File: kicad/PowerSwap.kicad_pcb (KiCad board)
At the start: 2 copper layers, 19 parts, among them U1 TPS63030

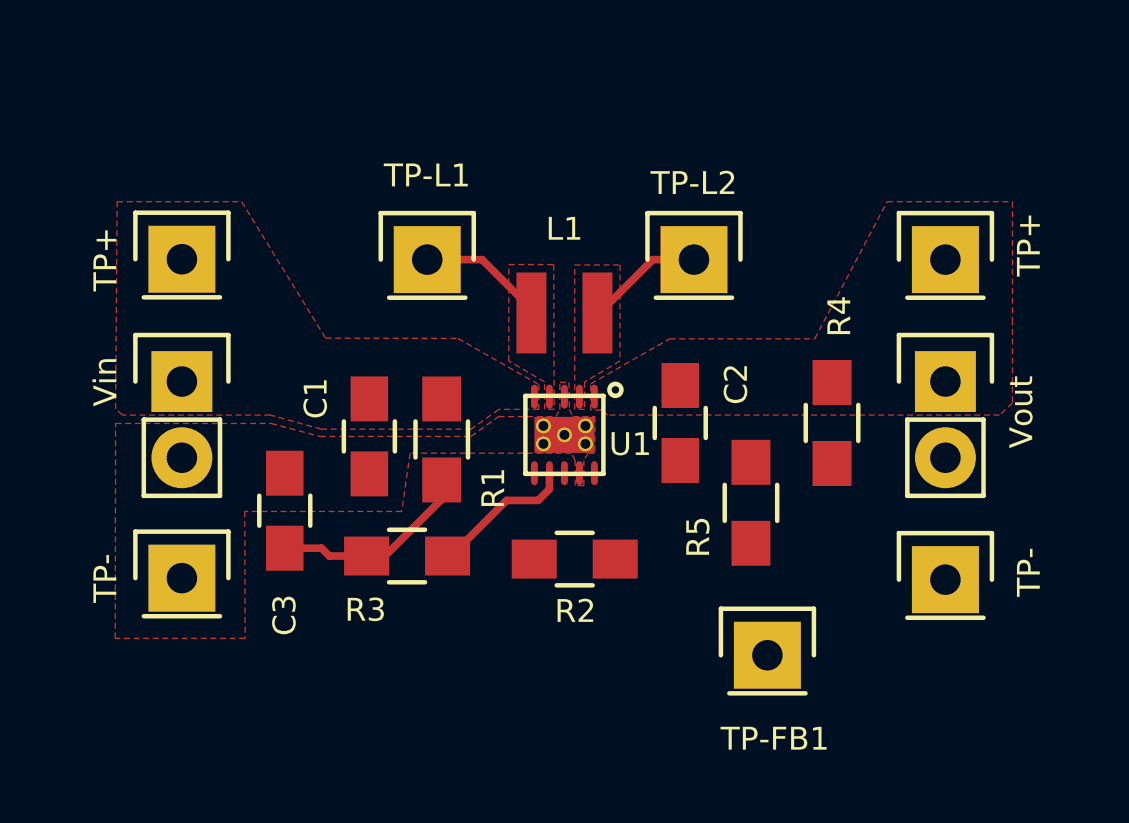
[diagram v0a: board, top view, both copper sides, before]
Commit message: Completed layout
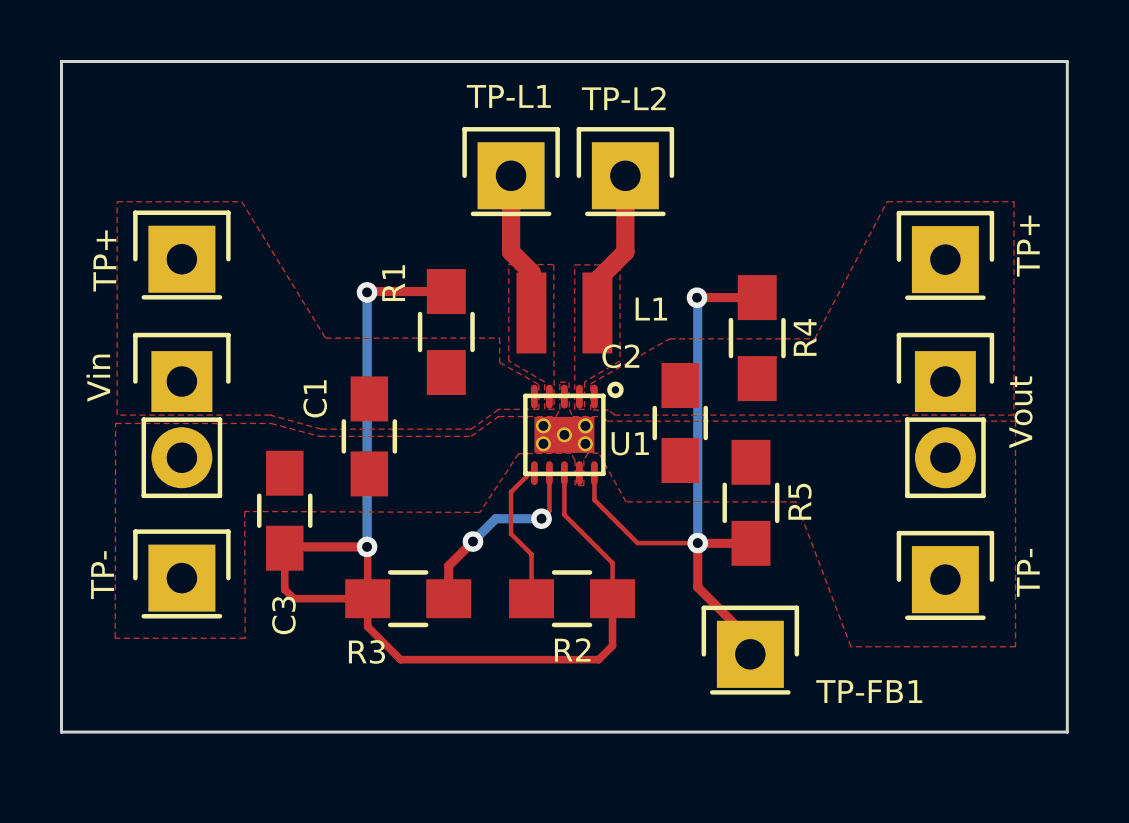
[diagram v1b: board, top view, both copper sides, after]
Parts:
- moved TP-L1 3.95 mm to (144.0, 86.1)
- moved R4 3.77 mm to (152.2, 91.5), turned to 90 degrees
- moved TP-L2 3.61 mm to (147.8, 86.1)
- moved R1 3.58 mm to (141.9, 91.3), turned to 270 degrees
- moved R3 1.42 mm to (140.6, 100.2)
- moved R2 1.32 mm to (146.1, 100.2)
- moved TP-FB1 0.57 mm to (152.0, 102.1)
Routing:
- net Net-(C3-Pad1): track 6.81 -> 36.3 mm, vias 0 -> 2
- net /Feedback: track 0.01 -> 21.4 mm, vias 0 -> 2
- net Net-(R2-Pad1): track 0.00 -> 4.89 mm
- net Net-(R3-Pad1): track 4.85 -> 6.47 mm, vias 0 -> 2
- net Net-(L1-Pad2): track 3.95 -> 5.03 mm
- net Net-(L1-Pad1): track 4.29 -> 5.05 mm
- added copper zone on B.Cu, net GNDPWR
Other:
- board outline added: 33.5 x 22.4 mm

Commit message: Final layout
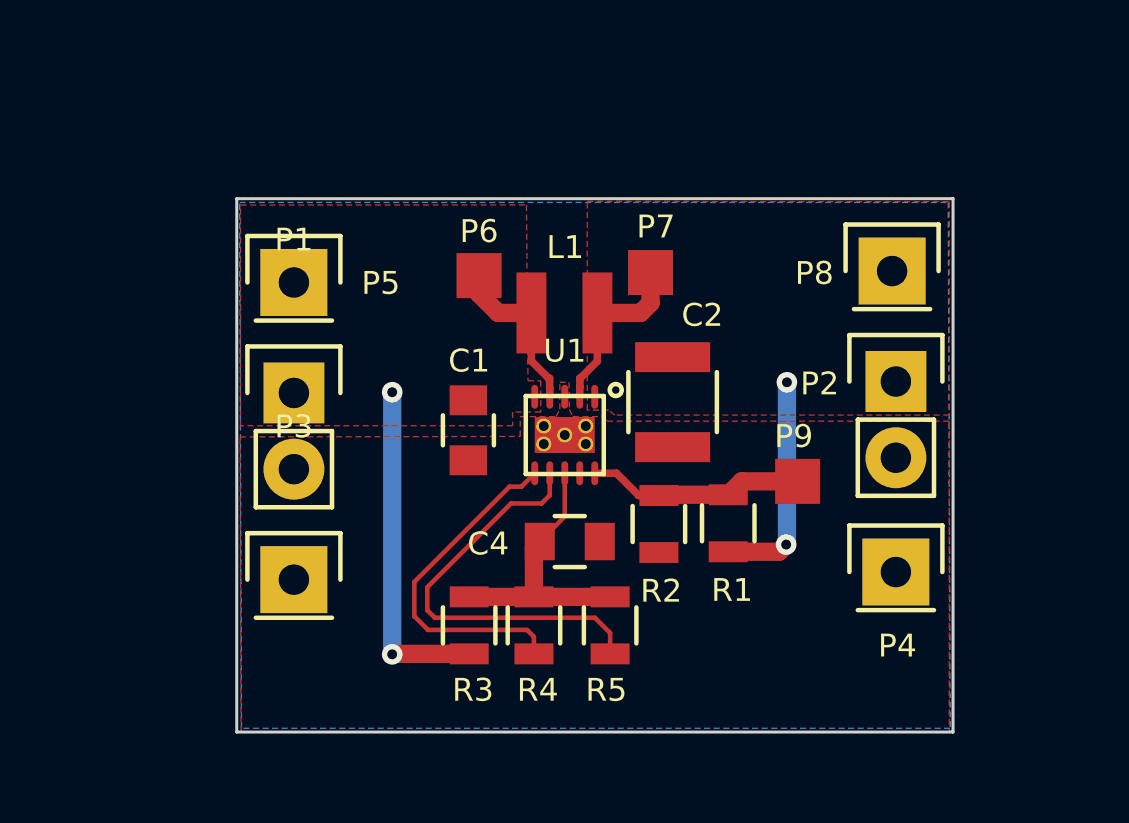
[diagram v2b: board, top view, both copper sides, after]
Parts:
- removed C3: 0.1μF, Capacitors_SMD:C_0805_HandSoldering
- removed TP+: Vin, Pin_Headers:Pin_Header_Straight_1x01
- removed TP+: Vout, Pin_Headers:Pin_Header_Straight_1x01
- removed TP-: GND, Pin_Headers:Pin_Header_Straight_1x01
- removed TP-: PGND, Pin_Headers:Pin_Header_Straight_1x01
- removed TP-FB1: Feedback, Pin_Headers:Pin_Header_Straight_1x01
- removed TP-L1: L1, Pin_Headers:Pin_Header_Straight_1x01
- removed TP-L2: L2, Pin_Headers:Pin_Header_Straight_1x01
- removed Vin: Battery, Pin_Headers:Pin_Header_Straight_1x02
- removed Vout: Vout, Pin_Headers:Pin_Header_Straight_1x02
- added C4: 0.1μF, Capacitors_SMD:C_0805, F.Cu at (146.0, 98.3)
- added P1: Battery, Pin_Headers:Pin_Header_Straight_1x02, F.Cu at (136.8, 93.3)
- added P2: Vout, Pin_Headers:Pin_Header_Straight_1x02, F.Cu at (156.8, 93.0)
- added P3: TST, Pin_Headers:Pin_Header_Straight_1x01, F.Cu at (136.8, 99.6)
- added P4: TST, Pin_Headers:Pin_Header_Straight_1x01, F.Cu at (156.8, 99.3)
- added P5: TST, Pin_Headers:Pin_Header_Straight_1x01, F.Cu at (136.8, 89.7)
- added P6: TST, Measurement_Points:Measurement_Point_Square-SMD-Pad_Small, F.Cu at (143.0, 89.4)
- added P7: TST, Measurement_Points:Measurement_Point_Square-SMD-Pad_Small, F.Cu at (148.7, 89.3)
- added P8: TST, Pin_Headers:Pin_Header_Straight_1x01, F.Cu at (156.7, 89.3)
- added P9: TST, Measurement_Points:Measurement_Point_Square-SMD-Pad_Small, F.Cu at (153.6, 96.3)
- C1: footprint Capacitors_SMD:C_0805_HandSoldering -> Capacitors_SMD:C_0805
- C2: value 11μF -> 22μF; footprint Capacitors_SMD:C_0805_HandSoldering -> Capacitors_SMD:C_1210
- R1: value 0 -> 2.1MΩ; footprint Resistors_SMD:R_0805_HandSoldering -> Resistors_SMD:R_0805
- R2: value 0 -> 215KΩ; footprint Resistors_SMD:R_0805_HandSoldering -> Resistors_SMD:R_0805
- R3: footprint Resistors_SMD:R_0805_HandSoldering -> Resistors_SMD:R_0805
- R4: value 2.1MΩ -> 0; footprint Resistors_SMD:R_0805_HandSoldering -> Resistors_SMD:R_0805
- R5: value 215KΩ -> 0; footprint Resistors_SMD:R_0805_HandSoldering -> Resistors_SMD:R_0805
- moved R4 12.1 mm to (144.8, 101.1)
- moved R1 11.4 mm to (151.3, 97.7), turned to 90 degrees
- moved R5 6.22 mm to (147.3, 101.1)
- moved R2 3.82 mm to (148.9, 97.7), turned to 270 degrees
- moved C1 3.31 mm to (142.6, 94.6)
- moved R3 2.22 mm to (142.6, 101.1), turned to 270 degrees
- moved C2 0.74 mm to (149.4, 93.6)
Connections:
- net Net-(L1-Pad1) renamed /L1
- net Net-(L1-Pad2) renamed /L2
- R1 pad 1: Net-(C3-Pad1) -> /Vout+
- R1 pad 2: /Vin+ -> /Feedback
- R2 pad 1: Net-(R2-Pad1) -> /Feedback
- R2 pad 2: Net-(C3-Pad1) -> GNDPWR
- R3 pad 1: Net-(R3-Pad1) -> /Vina
- R3 pad 2: Net-(C3-Pad1) -> /Vin+
- R4 pad 1: /Vout+ -> /EN
- R4 pad 2: /Feedback -> /Vina
- R5 pad 1: /Feedback -> /PS
- R5 pad 2: GNDPWR -> /Vina
- U1 pad 6: Net-(R2-Pad1) -> /EN
- U1 pad 7: Net-(R3-Pad1) -> /PS
- U1 pad 8: Net-(C3-Pad1) -> /Vina
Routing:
- net Net-(C3-Pad1): track 36.3 -> 0.00 mm, vias 2 -> 0
- net /Feedback: track 21.4 -> 7.26 mm, vias 2 -> 0
- net /PS: track 0.00 -> 14.0 mm
- net /EN: track 0.00 -> 11.5 mm
- net /Vin+: track 0.00 -> 11.3 mm, vias 0 -> 2
- net /Vina: track 0.00 -> 9.24 mm
- net /Vout+: track 0.00 -> 7.45 mm, vias 0 -> 2
- net Net-(R3-Pad1): track 6.47 -> 0.00 mm, vias 2 -> 0
- net Net-(R2-Pad1): track 4.89 -> 0.00 mm
- net /L2: track 5.03 -> 5.97 mm
- net /L1: track 5.05 -> 5.69 mm
- removed copper zone on F.Cu, net /L1
- removed copper zone on F.Cu, net /L2
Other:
- board size 33.5 x 22.4 mm -> 23.9 x 17.8 mm
